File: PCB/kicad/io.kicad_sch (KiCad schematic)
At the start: 64 parts, among them J10 CHEM 3, J11 FLOW, J12 HALL, J13 TEMP 1, J14 TEMP 2, J5 DISPLAY JP1, J6 C6 UART, J7 BATH LEVEL, J8 CHEM 1, J9 CHEM 2, U3 MCP23017-E/SS, U4 ADS1115

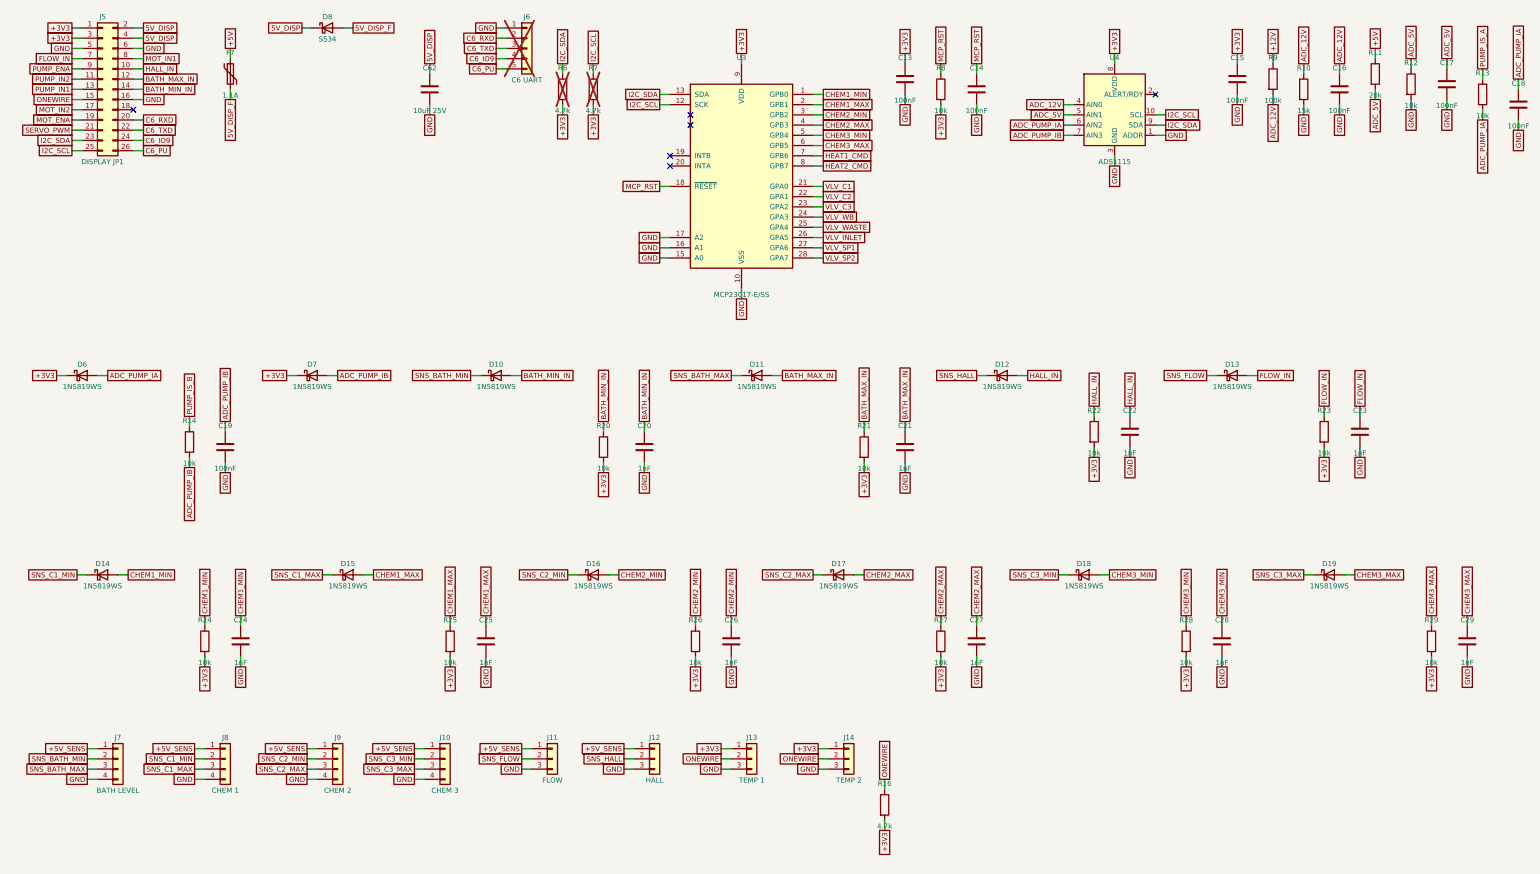
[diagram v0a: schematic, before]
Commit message: new pcb
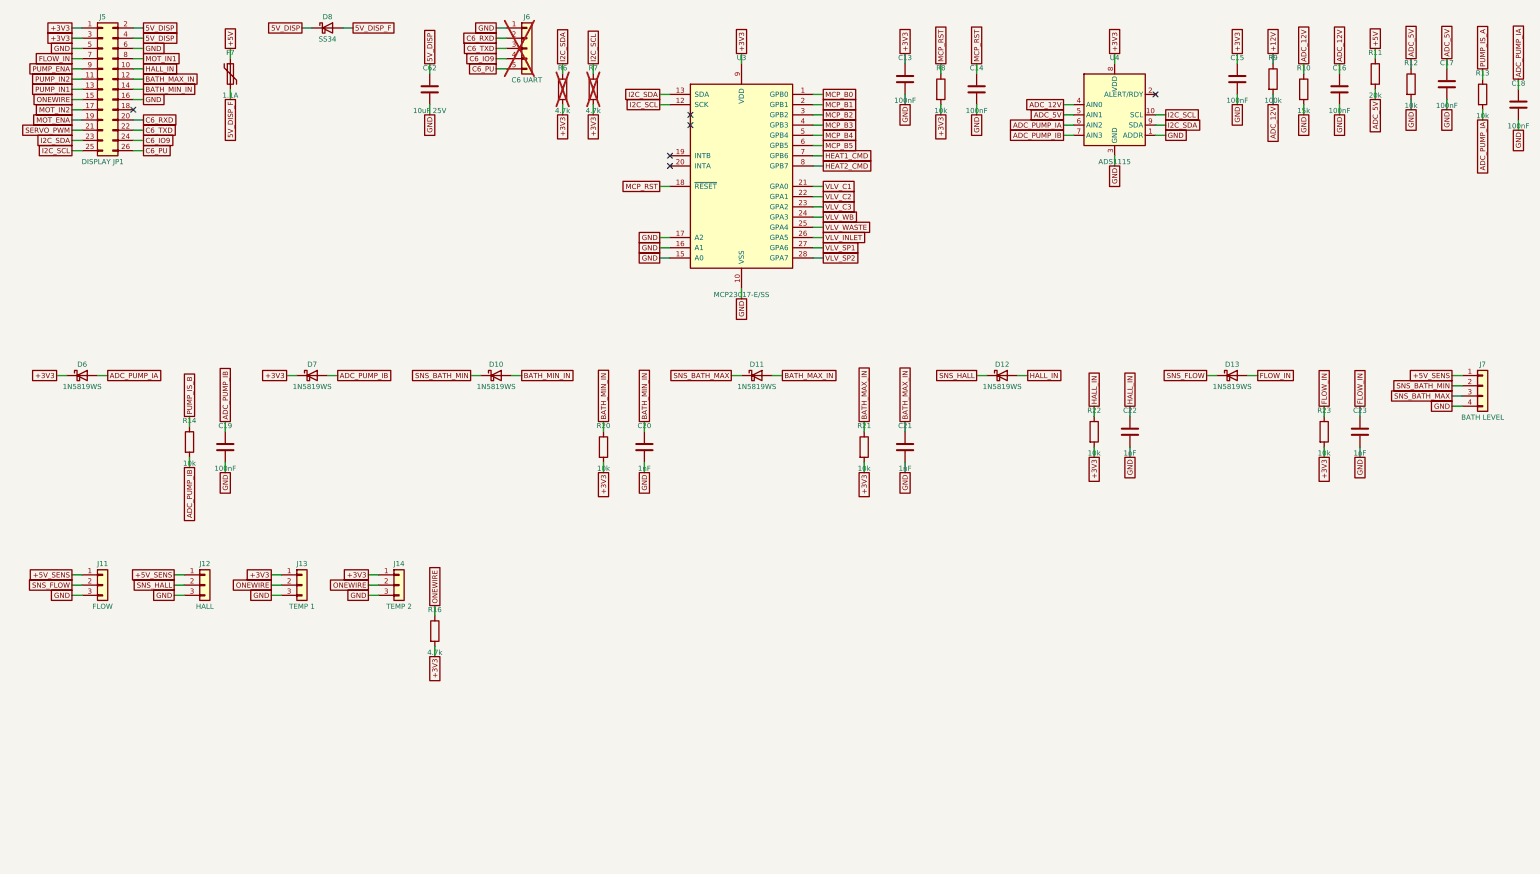
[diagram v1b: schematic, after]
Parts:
- removed C24, C25, C26, C27, C28, C29: 1nF, Capacitor_SMD:C_0603_1608Metric, symbol Device:C
- removed D15, D16, D17, D18, D19: 1N5819WS, Diode_SMD:D_SOD-323, symbol Device:D_Schottky
- removed J10: CHEM 3, Connector_JST:JST_XH_B4B-XH-A_1x04_P2.50mm_Vertical, symbol Connector_Generic:Conn_01x04
- removed J7: BATH LEVEL, Connector_JST:JST_XH_B4B-XH-A_1x04_P2.50mm_Vertical, symbol Connector_Generic:Conn_01x04
- removed J8: CHEM 1, Connector_JST:JST_XH_B4B-XH-A_1x04_P2.50mm_Vertical, symbol Connector_Generic:Conn_01x04
- removed J9: CHEM 2, Connector_JST:JST_XH_B4B-XH-A_1x04_P2.50mm_Vertical, symbol Connector_Generic:Conn_01x04
- removed R24, R25, R26, R27, R28, R29: 10k, Resistor_SMD:R_0603_1608Metric, symbol Device:R
- J7: renamed from D14; value 1N5819WS -> BATH LEVEL; footprint Diode_SMD:D_SOD-323 -> Connector_JST:JST_XH_B4B-XH-A_1x04_P2.50mm_Vertical; symbol Device:D_Schottky -> Connector_Generic:Conn_01x04; LCSC C191023 -> C37815; MPN 1N5819WS -> XH-4A; Manufacturer JLCPCB basic -> BOOMELE
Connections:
- net SNS_C1_MIN is gone; now on net +5V_SENS: J7.1 (Pin_1)
- net GND: now also J7.4 (Pin_4)
- net SNS_BATH_MAX: now also J7.3 (Pin_3)
- net SNS_BATH_MIN: now also J7.2 (Pin_2)
- net CHEM1_MAX renamed MCP_B1
- net CHEM1_MIN renamed MCP_B0
- net MCP_B0: no longer J7.2 (A)
- net CHEM2_MAX renamed MCP_B3
- net CHEM2_MIN renamed MCP_B2
- net CHEM3_MAX renamed MCP_B5
- net CHEM3_MIN renamed MCP_B4
